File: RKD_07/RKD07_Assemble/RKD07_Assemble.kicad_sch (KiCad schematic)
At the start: 160 parts, among them J1 Conn_01x02_Socket, J10 Conn_01x04, J11 TRRS, J12 Conn_01x06, J13 Conn_01x06, J2 Conn_01x24, J3 Conn_01x24, J4 Conn_01x24, J5 Qwiic_RA, J6 Qwiic_RA, J7 Conn_01x06, J8 Conn_01x06, J9 Conn_01x04, SW1 SW_Push, SW10 SW_Push, SW11 SW_Push, SW12 SW_Push, SW13 SW_Push, SW14 SW_Push, SW15 SW_Push, SW16 SW_Push, SW17 SW_Push, SW18 SW_Push, SW19 SW_Push, SW2 SW_Push, SW20 SW_Push, SW21 SW_Push, SW22 SW_Push, SW23 SW_Push, SW24 SW_Push, SW25 SW_Push, SW26 SW_Push, SW27 SW_Push, SW28 SW_Push, SW29 SW_Push, SW3 SW_Push, SW30 RotaryEncoder_Switch, SW31 SW_Push, SW4 SW_Push, SW5 SW_Push, SW51 SW_Push, SW52 SW_Push, SW53 SW_Push, SW54 SW_Push, SW55 SW_Push, SW56 SW_Push, SW57 SW_Push, SW58 SW_Push, SW59 SW_Push, SW6 SW_Push, SW60 SW_Push, SW61 SW_Push, SW62 SW_Push, SW63 SW_Push, SW64 SW_Push, SW65 SW_Push, SW66 SW_Push, SW67 SW_Push, SW68 SW_Push, SW69 SW_Push, SW7 SW_Push, SW70 SW_Push, SW71 SW_Push, SW72 SW_Push, SW73 SW_Push, SW74 SW_Push, SW75 SW_Push, SW76 SW_Push, SW77 SW_Push, SW78 SW_Push, SW79 SW_Push, SW8 SW_Push, SW80 SW_Push, SW81 SW_Push, SW82 SW_Push, SW83 SW_Push, SW84 SW_Push, SW85 SW_Push, SW86 SW_Push, SW87 SW_Push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

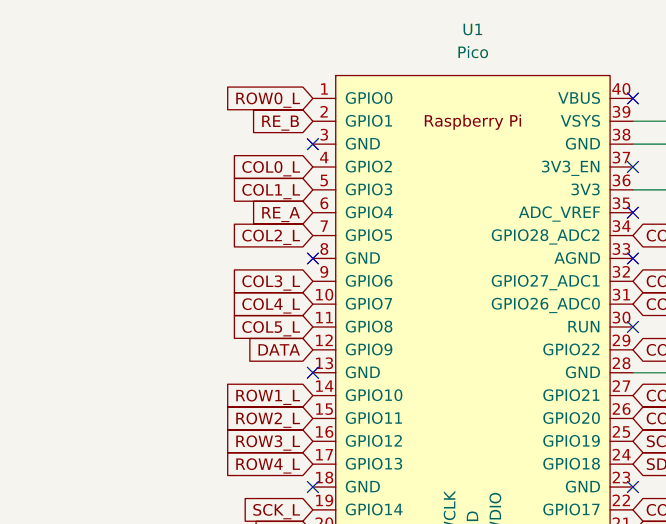
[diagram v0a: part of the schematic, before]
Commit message: QWICC位置など調整
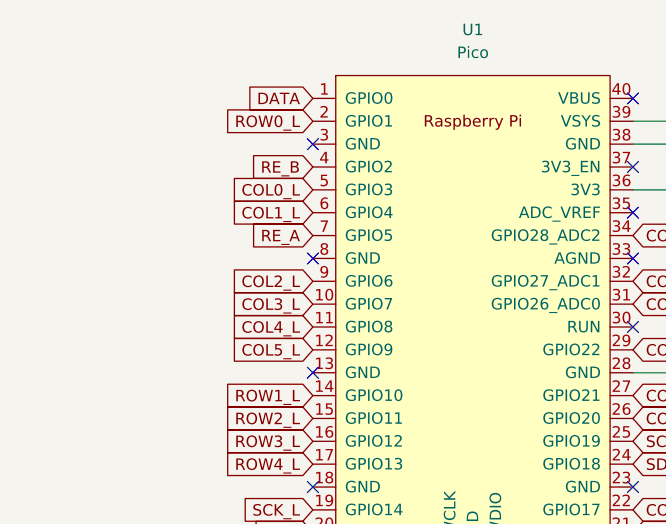
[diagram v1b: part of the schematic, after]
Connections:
- net COL0_L: now also U1.5 (GPIO3); no longer U1.4 (GPIO2)
- net COL1_L: now also U1.6 (GPIO4); no longer U1.5 (GPIO3)
- net COL2_L: now also U1.9 (GPIO6); no longer U1.7 (GPIO5)
- net COL3_L: now also U1.10 (GPIO7); no longer U1.9 (GPIO6)
- net COL4_L: now also U1.11 (GPIO8); no longer U1.10 (GPIO7)
- net COL5_L: now also U1.12 (GPIO9); no longer U1.11 (GPIO8)
- net DATA: now also U1.1 (GPIO0); no longer U1.12 (GPIO9)
- net RE_A: now also U1.7 (GPIO5); no longer U1.6 (GPIO4)
- net RE_B: now also U1.4 (GPIO2); no longer U1.2 (GPIO1)
- net ROW0_L: now also U1.2 (GPIO1); no longer U1.1 (GPIO0)
